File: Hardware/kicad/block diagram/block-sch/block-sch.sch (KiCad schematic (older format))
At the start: 14 parts

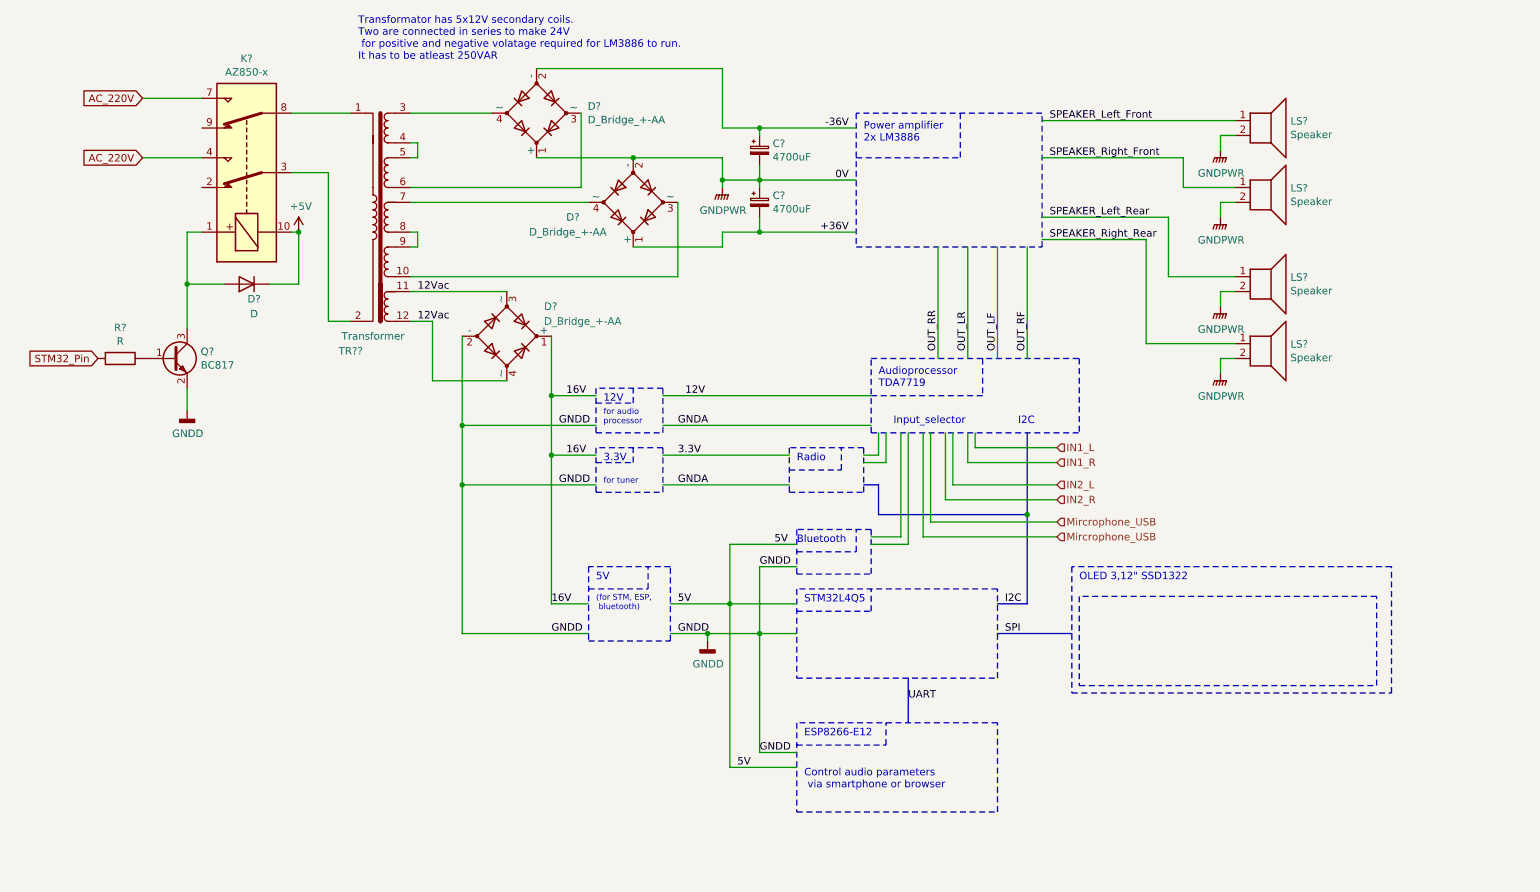
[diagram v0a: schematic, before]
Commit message: new
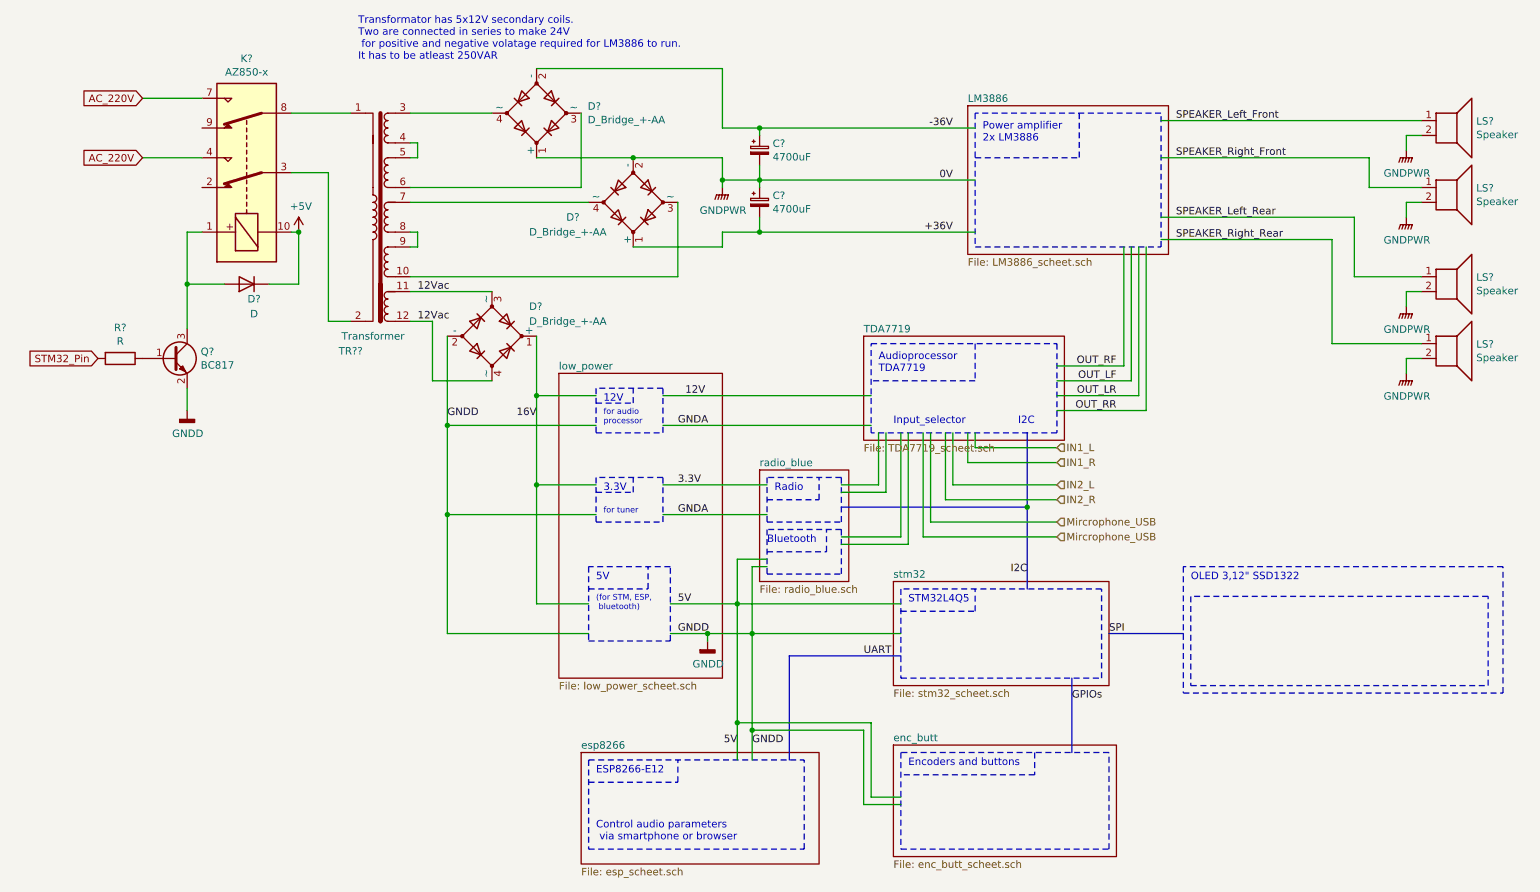
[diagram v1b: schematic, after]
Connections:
- net labels added: GPIOs
- wire segments 120 -> 130
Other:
- note added: "Encoders and buttons"
- moved on the sheet: D?, LS?
